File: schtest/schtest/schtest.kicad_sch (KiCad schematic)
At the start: 6 parts, among them P1 RZM001P02T2L, P2 RZM001P02T2L

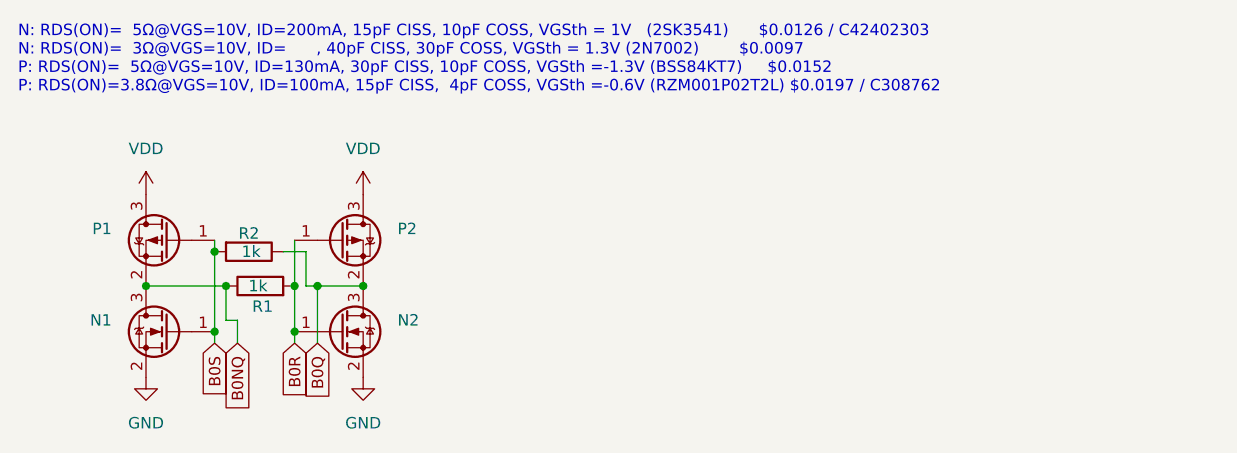
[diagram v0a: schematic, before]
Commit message: Cleanup schematic
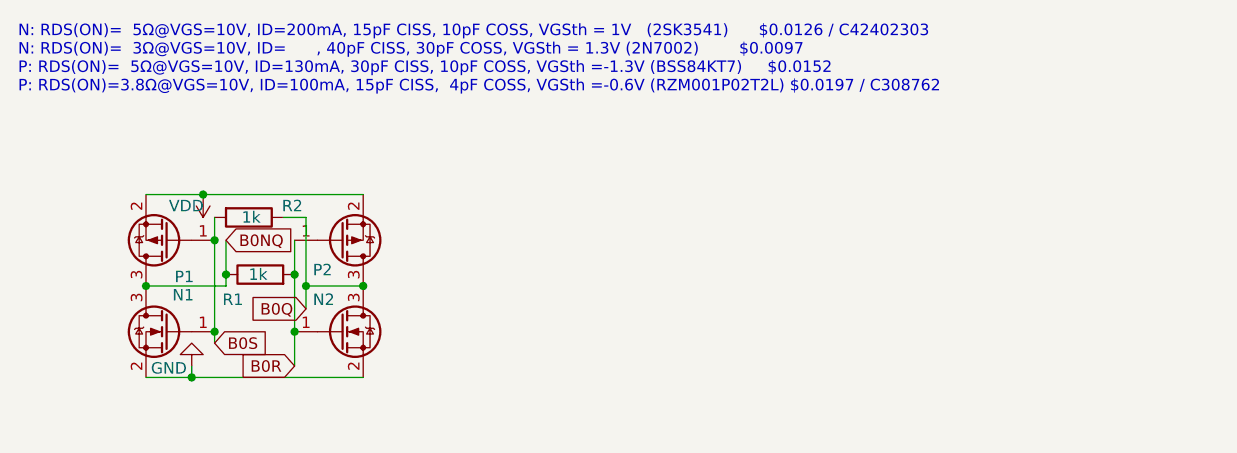
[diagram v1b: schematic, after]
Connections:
- net B0NQ: now also P1.3 (D); no longer P1.2 (S)
- net B0Q: now also P2.3 (D); no longer P2.2 (S)
- net VDD: now also P1.2 (S), P2.2 (S); no longer P1.3 (D), P2.3 (D)
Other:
- moved on the sheet: P1, R1, R2
